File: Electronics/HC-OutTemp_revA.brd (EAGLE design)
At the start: 80 x 80 mm, 38 parts, among them Q1 16MHz, SW1 SWITCH_SLIDE, U1 ATMEGA328-20P, U2 NRF24L01, U5 BCO35

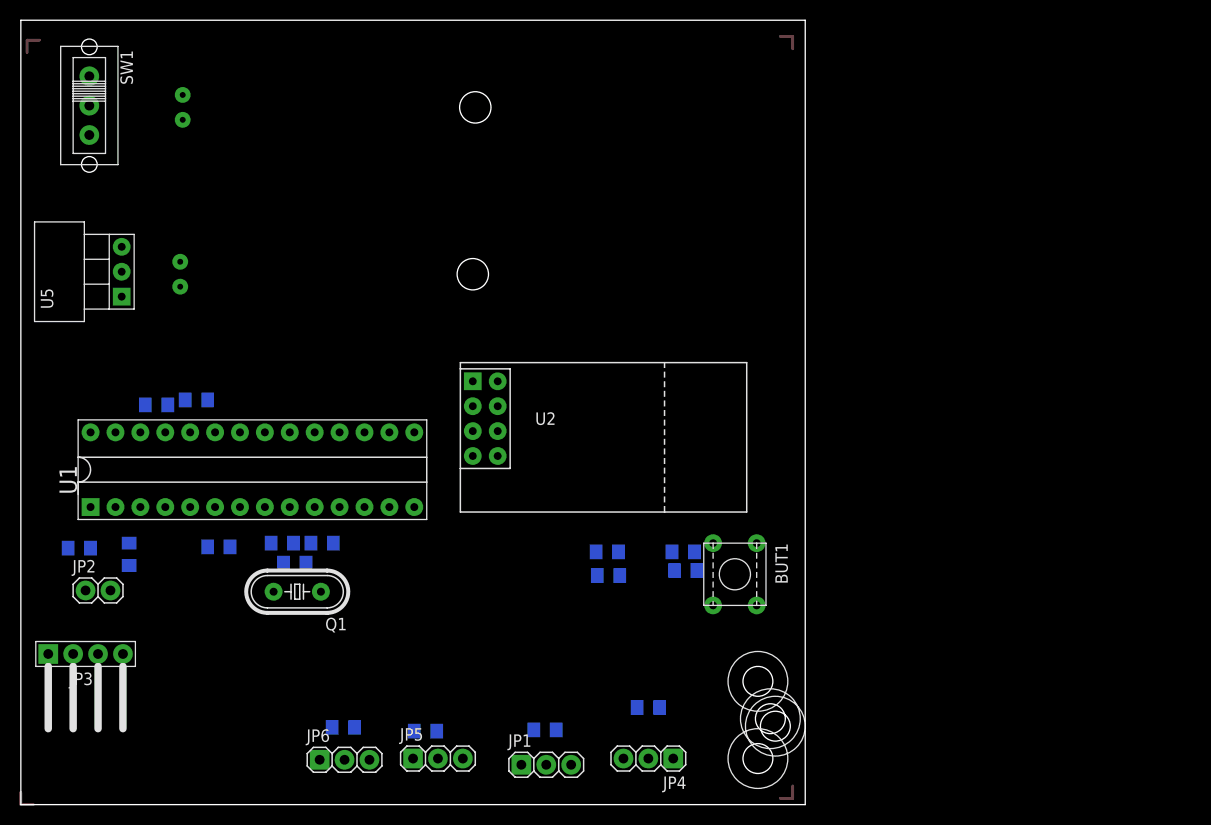
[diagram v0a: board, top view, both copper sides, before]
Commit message: changed: PCB
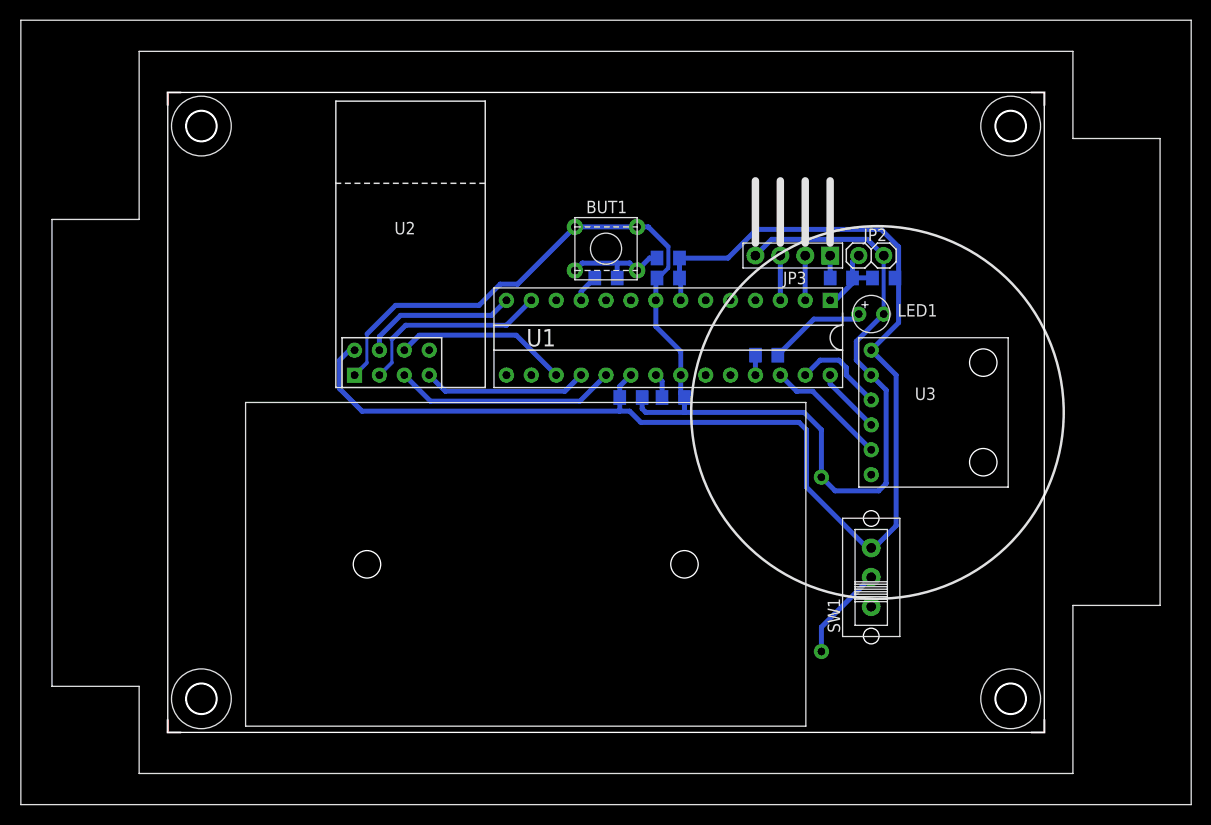
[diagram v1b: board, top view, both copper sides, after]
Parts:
- removed BAT2: 1V5, 1_domaci:1XAA_BATTERY_HOLDER
- removed C2, C3: 22p, 1_domaci:C0805
- removed JP1, JP4, JP5, JP6: PINHD-3X1, 1_domaci:PINHD-3X1
- removed Q1: 16MHz, crystal:HC49/S
- removed R10, R2, R3, R7: 4K7, 1_domaci:R0805
- removed R4: 1M, 1_domaci:R0805
- removed U5: BCO35, 1_domaci:BCO35
- added U$9: CASE'120X80X40', 1_domaci:CASE-120X80X40
- added U3: TMP102, 1_domaci:TMP102
- BAT1: value 1V5 -> (none); device 1_domaci:1XAA_BATTERY_HOLDER -> 1_domaci:2XAA_BATTERY_HOLDER
- LED1: value green -> (none); device 1_domaci:LED0805 -> 1_domaci:LED3MM
- moved SW1 93.2 mm to (86.7, 23.1), turned to 90 degrees
- moved R1 86.5 mm to (88.0, 53.7), turned to 180 degrees
- moved JP2 85.9 mm to (86.7, 56.0), turned to 180 degrees
- moved U$7 84.7 mm to (18.4, 69.2)
- moved JP3 82.8 mm to (78.7, 56.0), turned to 0 degrees
- moved C4 77.9 mm to (83.7, 53.7), turned to 0 degrees
- moved U$5 69.5 mm to (101.0, 69.2)
- moved U$8 58.1 mm to (18.4, 10.8)
- moved C1 53.4 mm to (66.0, 53.7), turned to 180 degrees
- moved C5 48.6 mm to (66.5, 41.5), turned to 180 degrees
- moved C6 48.4 mm to (62.2, 41.5)
- moved U1 44.5 mm to (66.0, 47.6), turned to 180 degrees
- moved LED1 37.8 mm to (86.7, 50.0), flipped to the top, turned to 0 degrees
- moved BUT1 35.8 mm to (59.1, 57.0), turned to 0 degrees
- moved R6 30.9 mm to (59.7, 53.7)
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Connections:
- removed net DS18B20_1: JP4.2, R10.1, U1.13
- removed net DS18B20_2: JP1.2, R2.1, U1.14
- removed net DS18B20_3: JP5.2, R3.1, U1.15
- removed net DS18B20_4: JP6.2, R7.1, U1.16
- removed net N$11: LED1.1, R9.1
- removed net N$4: C2.2, Q1.2, R4.2, U1.9
- removed net N$8: BAT1.P, BAT2.P, SW1.2
- removed net V_BAT: SW1.3, U1.23, U5.IN
- new net N$10: U1.28, U3.SCL
- new net N$12: U1.26, U3.ALT
- new net N$3: LED1.A, R9.1
- new net N$9: U1.27, U3.SDA
- net +3V3: now also SW1.3, U3.VCC; no longer JP1.1, JP4.1, JP5.1, JP6.1, R10.2, R2.2, R3.2, R7.2, U5.OUT
- net BUT: now also U1.11; no longer U1.4
- net CE_R: now also U1.13; no longer U1.24
- net CS_R: now also U1.14; no longer U1.25
- net GND: now also LED1.K, U3.GND; no longer BAT2.N, C2.1, C3.1, JP1.3, JP4.3, JP5.3, JP6.3, LED1.2, U5.GND
- net LED: now also U1.25; no longer U1.5
- net N$1: now also BAT1.P, SW1.2; no longer C3.2, Q1.1, R4.1, U1.10
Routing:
- net +3V3: track 0.00 -> 136.7 mm
- net GND: track 0.00 -> 132.3 mm
- net SCK: track 0.00 -> 22.8 mm
- net CE_R: track 0.00 -> 20.1 mm
- net MOSI: track 0.00 -> 17.8 mm
- net MISO: track 0.00 -> 16.9 mm
- net CS_R: track 0.00 -> 15.9 mm
- net N$12: track 0.00 -> 12.4 mm
- net N$7: track 0.00 -> 11.1 mm
- net N$3: track 0.00 -> 10.1 mm
- net N$1: track 0.00 -> 9.67 mm
- net N$9: track 0.00 -> 9.49 mm
- net N$2: track 0.00 -> 8.11 mm
- net N$10: track 0.00 -> 6.82 mm
- net TX: track 0.00 -> 4.57 mm
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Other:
- board size 80 x 80 mm -> 89.4 x 65.3 mm
